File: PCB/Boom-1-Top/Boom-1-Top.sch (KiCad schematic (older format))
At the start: 983 parts, among them J1 DEBUG, J10 PIC_DEBUG, J11 PIC_DEBUG, J12 PIC_DEBUG, J13 PIC_DEBUG, J14 PIC_DEBUG, J15 USB_B_Micro, J16 SD_Card, J17 BT_DEBUG, J18 12V Supply, J19 3V3 Bypass, J2 MIDI IN, J20 5V Bypass, J21 Env +12V Supply, J22 Env -12V Supply, J23 OLEDConn, J3 MIDI OUT, J37 Osc1Conn, J38 Osc2Conn, J39 SubNoiseConn, J4 PIC_DEBUG, J40 FiltConn2, J41 EnvGenConn2, J42 EnvGenConn1, J43 FXConn1, J44 FiltConn1, J45 FXConn2, J46 EnvGenConn3, J5 PIC_DEBUG, J6 PIC_DEBUG, J7 PIC_DEBUG, J8 PIC_DEBUG, J9 PIC_DEBUG, Q1 AO3401A, Q2 AO3401A, SW1 Osc1SawEncoder, SW10 SubToOsc2FiltEncoder, SW11 Osc1ToOsc2FiltEncoder, SW12 Osc1FiltFreqEncoder, SW13 Osc2FiltFreqEncoder, SW14 SubFiltFreqEncoder, SW15 OscFiltEnvAttackEncoder, SW16 SubFiltEnvAttackEncoder, SW17 Osc1FiltResEncoder, SW18 Osc2FiltResEncoder, SW19 SubFiltResEncoder, SW2 Osc1SqrEncoder, SW20 OscFiltEnvDecayEncoder, SW21 SubFiltEnvDecayEncoder, SW22 OscFiltEnvSustainEncoder, SW23 SubFiltEnvSustainEncoder, SW24 Osc1DriveEncoder, SW25 Osc2DistortionEncoder, SW26 OscFiltEnvReleaseEncoder, SW27 SubFiltEnvReleaseEncoder, SW28 FXWetDryEncoder, SW29 SubAmpEnvAttackEncoder, SW3 Rotary_Encoder, SW30 OscAmpEnvAttackEncoder, SW31 FXControl1Encoder, SW32 SubAmpEnvDecayEncoder, SW33 OscAmpEnvDecayEncoder, SW34 FXControl2Encoder, SW35 SubAmpEnvSustainEncoder, SW36 OscAmpEnvSustainEncoder, SW37 FXControl3Encoder, SW38 FXFeedbackEncoder, SW39 SubAmpEnvReleaseEncoder, SW4 Rotary_Encoder_Switch, SW40 OscAmpEnvReleaseEncoder, SW41 Reset, SW42 SW_Push, SW43 Reset, SW44 SW_Push, SW45 SW_Push, SW46 SW_Push, SW47 SW_Push, SW48 SW_Push, SW49 SW_Push, SW5 Rotary_Encoder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

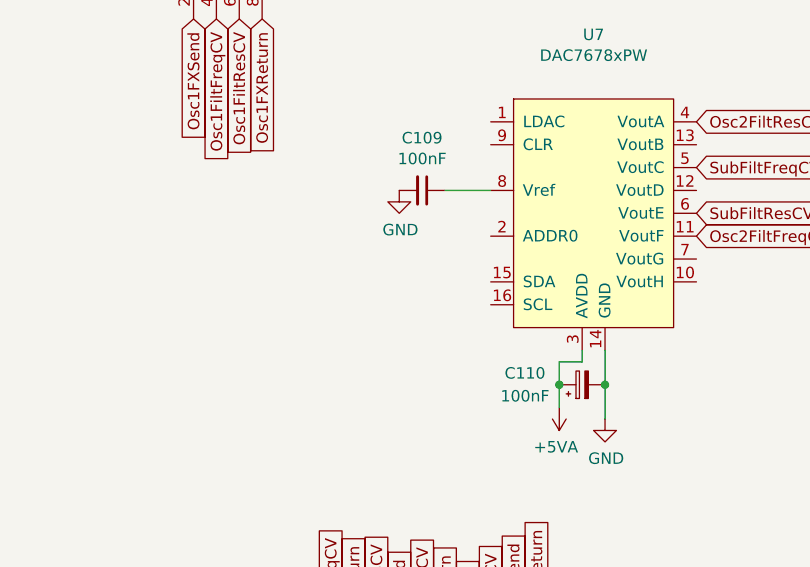
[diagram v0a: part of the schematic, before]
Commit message: U7 DAC i2c
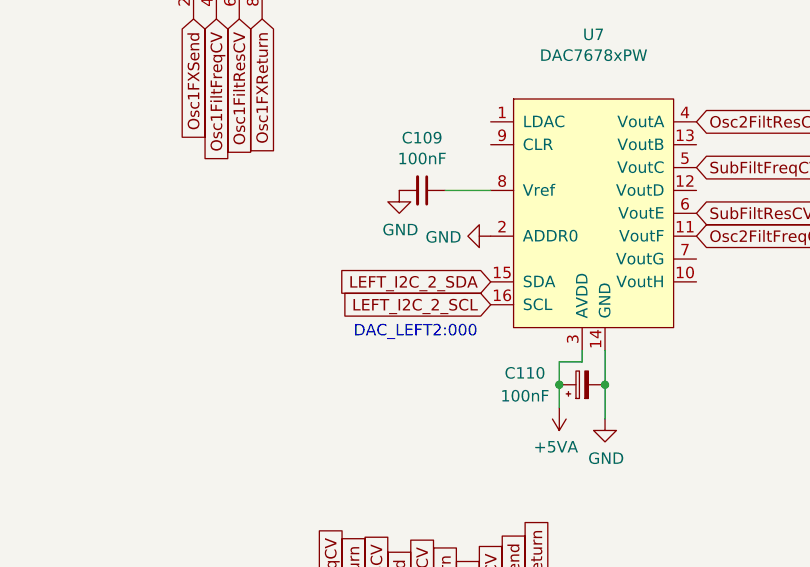
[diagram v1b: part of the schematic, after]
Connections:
- net GND: now also U7.2 (ADDR0)
- net LEFT_I2C_2_SCL: now also U7.16 (SCL)
- net LEFT_I2C_2_SDA: now also U7.15 (SDA)
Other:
- note added: "DAC_LEFT2:000"
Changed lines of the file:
@@
 LEFT_I2C_0_SCL
 $Comp
-L power:+5VA #PWR?
+L power:+5VA #PWR0925
 U 1 1 61BE5A1B
 P 29500 43400
-F 0 "#PWR?" H 29500 43250 50  0001 C CNN
+F 0 "#PWR0925" H 29500 43250 50  0001 C CNN
 F 1 "+5VA" V 29515 43527 50  0000 L CNN
 F 2 "" H 29500 43400 50  0001 C CNN
@@
 	0    -1   -1   0
 $EndComp
+Text Notes 32900 40050 0    50   ~ 0
+DAC_LEFT2:000
+Text GLabel 33500 39800 0    50   Input ~ 0
+LEFT_I2C_2_SDA
+Text GLabel 33500 39900 0    50   Input ~ 0
+LEFT_I2C_2_SCL
+$Comp
+L power:GND #PWR?
+U 1 1 626D0E19
+P 33500 39600
+F 0 "#PWR?" H 33500 39350 50  0001 C CNN
+F 1 "GND" V 33505 39472 50  0000 R CNN
+F 2 "" H 33500 39600 50  0001 C CNN
+F 3 "" H 33500 39600 50  0001 C CNN
+	1    33500 39600
+	0    1    1    0
+$EndComp
 $EndSCHEMATC
